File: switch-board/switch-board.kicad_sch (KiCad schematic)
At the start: 16 parts

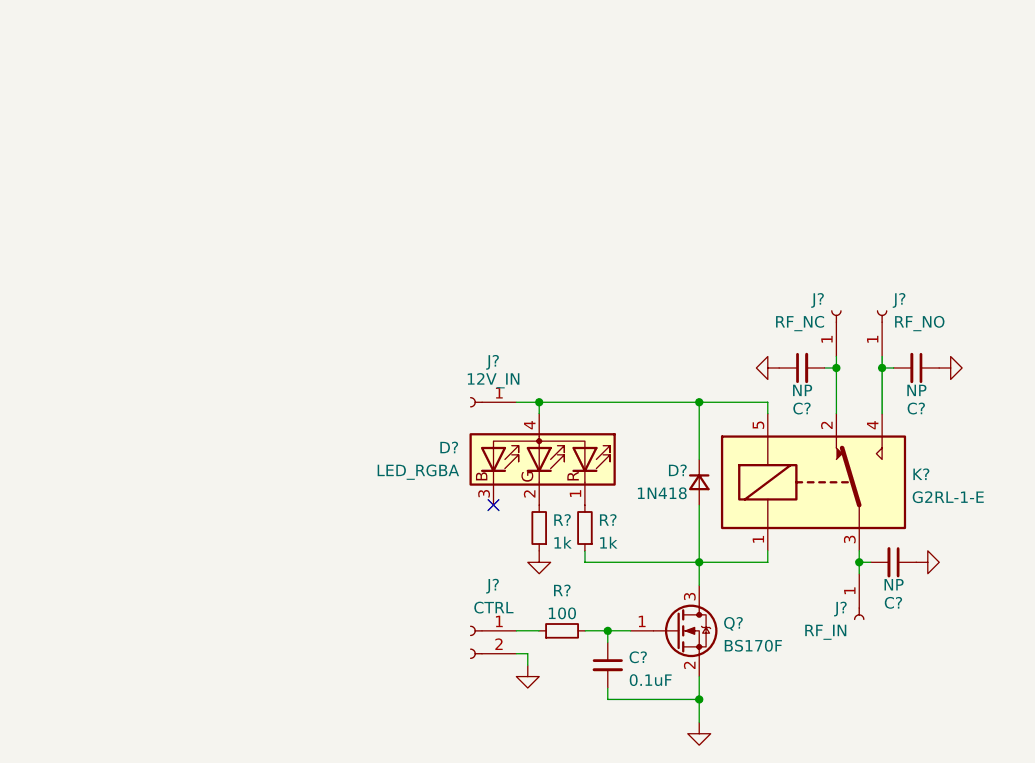
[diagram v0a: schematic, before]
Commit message: finalized rev A PCB
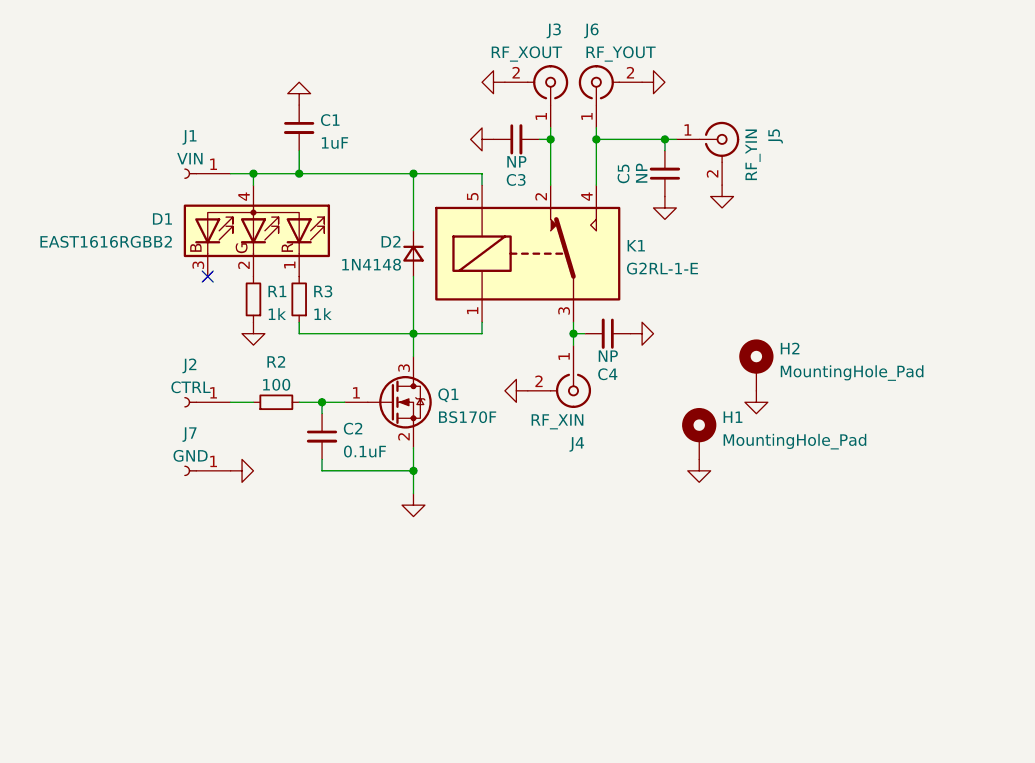
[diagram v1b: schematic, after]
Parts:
- removed J?: 12V_IN, symbol Connector:Conn_01x01_Female
- removed J?: RF_NO, symbol Connector:Conn_01x01_Female
- removed J?: RF_IN, symbol Connector:Conn_01x01_Female
- removed J?: CTRL, symbol Connector:Conn_01x02_Female
- removed J?: RF_NC, symbol Connector:Conn_01x01_Female
- added C1: 1uF, Capacitor_SMD:C_0805_2012Metric_Pad1.18x1.45mm_HandSolder, symbol Device:C_Small
- added H1, H2: MountingHole_Pad, MountingHole:MountingHole_4.3mm_M4_Pad, symbol Mechanical:MountingHole_Pad
- added J1: VIN, TestPoint:TestPoint_Pad_1.5x1.5mm, symbol Connector:Conn_01x01_Female
- added J2: CTRL, TestPoint:TestPoint_Pad_1.5x1.5mm, symbol Connector:Conn_01x01_Female
- added J3: RF_XOUT, conn:Coax_Edge_2.54_1.27, symbol Connector:Conn_Coaxial
- added J4: RF_XIN, conn:Coax_Edge_2.54_1.27, symbol Connector:Conn_Coaxial
- added J5: RF_YIN, conn:Coax_Edge_2.54_1.27, symbol Connector:Conn_Coaxial
- added J6: RF_YOUT, conn:Coax_Edge_2.54_1.27, symbol Connector:Conn_Coaxial
- added J7: GND, TestPoint:TestPoint_Pad_1.5x1.5mm, symbol Connector:Conn_01x01_Female
- C2: renamed from C?; footprint (none) -> Capacitor_SMD:C_0805_2012Metric_Pad1.18x1.45mm_HandSolder
- C3, C4, C5: renamed from C?; footprint (none) -> Capacitor_SMD:C_1812_4532Metric_Pad1.57x3.40mm_HandSolder
- D1: renamed from D?; value LED_RGBA -> EAST1616RGBB2; footprint (none) -> led:LED_SMD_1616_RGBA
- D2: renamed from D?; value 1N418 -> 1N4148; footprint (none) -> Diode_SMD:D_SOD-323_HandSoldering
- R1, R2, R3: renamed from R?; footprint (none) -> Resistor_SMD:R_0805_2012Metric_Pad1.20x1.40mm_HandSolder
- gave numbers to parts that had none: 2
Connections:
- net GND: now also C1.1, H1.1, H2.1, J3.2 (Ext), J4.2 (Ext), J5.2 (Ext), J6.2 (Ext), J7.1 (Pin_1)
- net at C5.2, K1.4: now also J5.1 (In), J6.1 (In)
- net at D1.4 (A), D2.1 (K), K1.5: now also C1.2, J1.1 (Pin_1)
- net at C3.2, K1.2: now also J3.1 (In)
- net at C4.2, K1.3: now also J4.1 (In)
- net at R2.1: now also J2.1 (Pin_1)
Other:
- moved on the sheet: C2, C3, C4, C5, D1, D2, K1, Q1, R1, R2, R3
